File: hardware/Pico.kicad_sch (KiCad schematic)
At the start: 36 parts, among them J1 Conn_01x03 2.54mm, J5 Conn_01x04, J6 Conn_01x06, J7 Conn_01x12, U10 SRV05-4, U6 SRV05-4, U7 SRV05-4, U9 SRV05-4

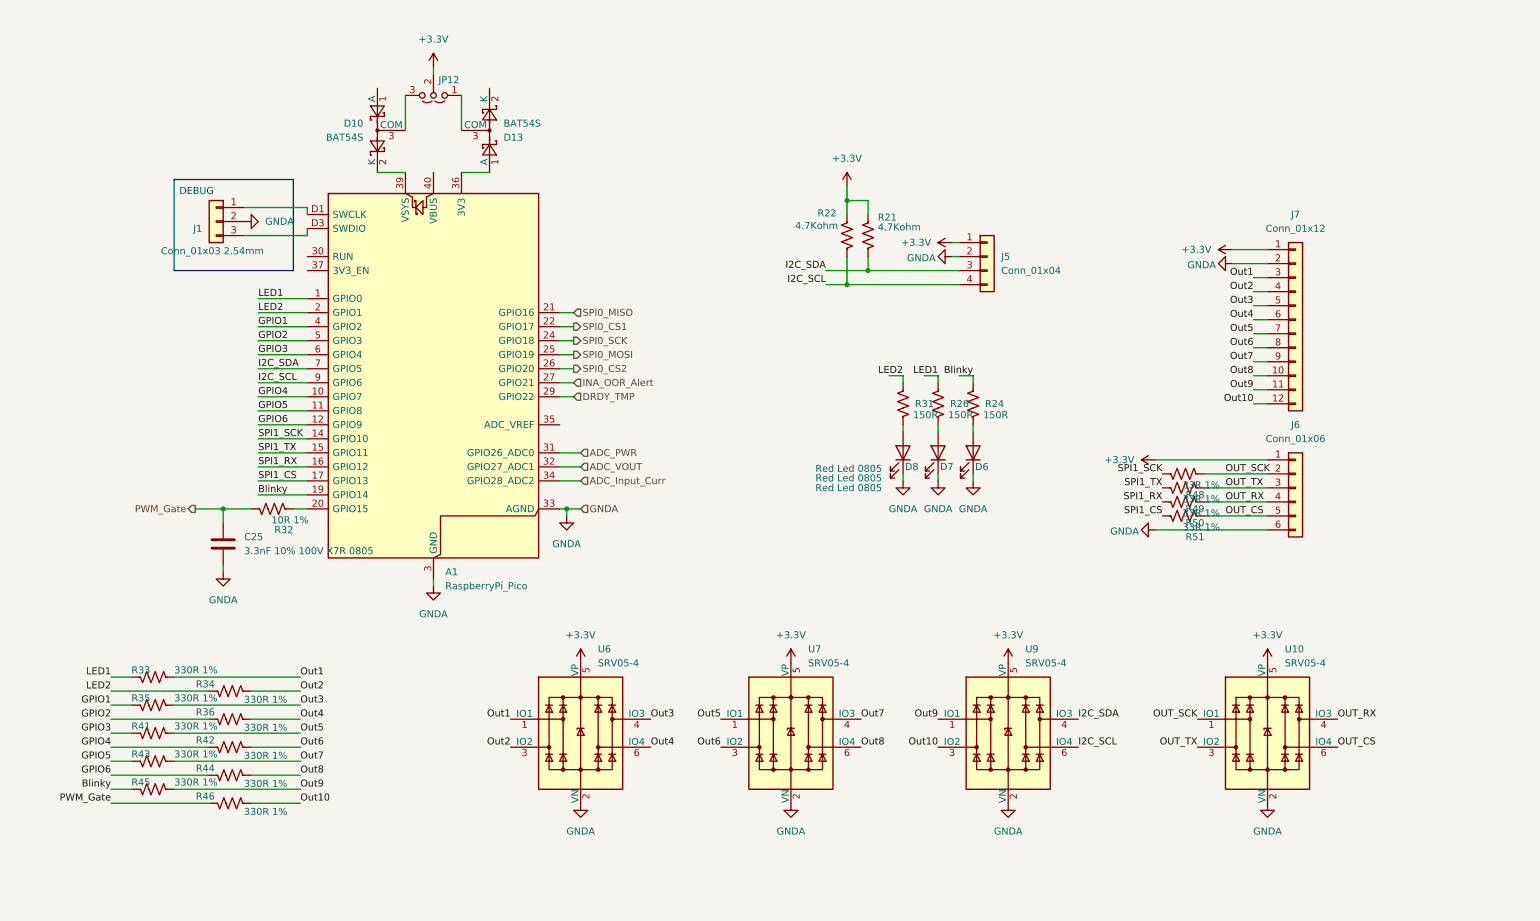
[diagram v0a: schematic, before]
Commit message: Hw/placa sepic (#34)
Co-authored-by: Federico Borello <156438142+fborello-lambda@users.noreply.github.com>
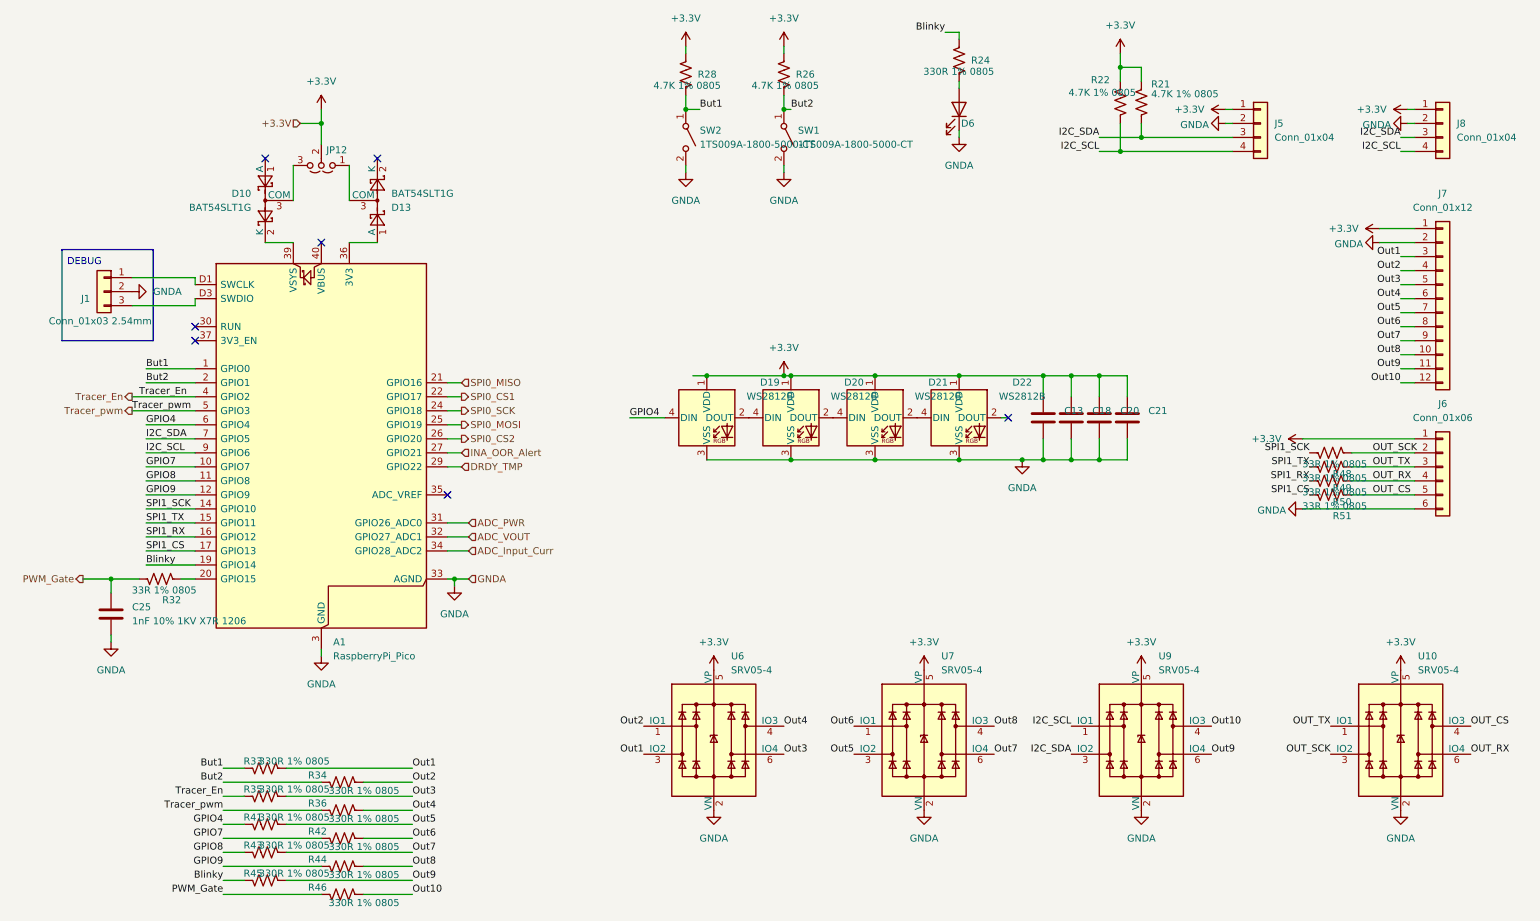
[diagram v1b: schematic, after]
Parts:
- removed D7, D8: Red Led 0805, LED_SMD:LED_0805_2012Metric_Pad1.15x1.40mm_HandSolder, symbol Device:LED
- removed R31: 150R, Resistor_SMD:R_0805_2012Metric_Pad1.20x1.40mm_HandSolder, symbol Device:R_US
- added C13, C18, C20, C21: 100nF 10% 50V X7R 0805, Capacitor_SMD:C_0805_2012Metric, symbol Device:C
- added D19, D20, D21, D22: WS2812B, LED_SMD:LED_WS2812B_PLCC4_5.0x5.0mm_P3.2mm, symbol LED:WS2812B
- added J8: Conn_01x04, Connector_PinHeader_2.54mm:PinHeader_1x04_P2.54mm_Vertical, symbol Connector_Generic:Conn_01x04
- added R28: 4.7K 1% 0805, Resistor_SMD:R_0805_2012Metric, symbol Device:R_US
- added SW1, SW2: 1TS009A-1800-5000-CT, Button_Switch_SMD:SW_Push_1TS009xxxx-xxxx-xxxx_6x6x5mm, symbol Switch:SW_SPST
- C25: value 3.3nF 10% 100V X7R 0805 -> 1nF 10% 1KV X7R 1206; footprint Capacitor_SMD:C_0805_2012Metric_Pad1.18x1.45mm_HandSolder -> Capacitor_SMD:C_1206_3216Metric
- D10, D13: value BAT54S -> BAT54SLT1G
- D6: value Red Led 0805 -> YLED0805 Red; footprint LED_SMD:LED_0805_2012Metric_Pad1.15x1.40mm_HandSolder -> LED_SMD:LED_0805_2012Metric; LCSC Part C19171391 -> (none)
- J1, JP12: LCSC Part C42431836 -> (none)
- R21, R22: value 4.7Kohm -> 4.7K 1% 0805; footprint Resistor_SMD:R_0805_2012Metric_Pad1.20x1.40mm_HandSolder -> Resistor_SMD:R_0805_2012Metric; LCSC Part C153298 -> (none)
- R24: value 150R -> 330R 1% 0805; footprint Resistor_SMD:R_0805_2012Metric_Pad1.20x1.40mm_HandSolder -> Resistor_SMD:R_0805_2012Metric; LCSC Part C153298 -> (none)
- R26: value 150R -> 4.7K 1% 0805; footprint Resistor_SMD:R_0805_2012Metric_Pad1.20x1.40mm_HandSolder -> Resistor_SMD:R_0805_2012Metric; LCSC Part C153298 -> (none)
- R32: value 10R 1% -> 33R 1% 0805; footprint Resistor_SMD:R_0805_2012Metric_Pad1.20x1.40mm_HandSolder -> Resistor_SMD:R_0805_2012Metric
- R33, R34, R35, R36, R41, R42, R43, R44, R45, R46: value 330R 1% -> 330R 1% 0805; footprint Resistor_SMD:R_0805_2012Metric_Pad1.20x1.40mm_HandSolder -> Resistor_SMD:R_0805_2012Metric
- R48, R49, R50, R51: value 33R 1% -> 33R 1% 0805; footprint Resistor_SMD:R_0805_2012Metric_Pad1.20x1.40mm_HandSolder -> Resistor_SMD:R_0805_2012Metric
- U10, U6, U7, U9: LCSC Part (none) -> C1975211
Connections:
- net GPIO3 is gone; now on net GPIO4: A1.6 (GPIO4), R41.1
- net LED2 is gone; now on net But2: A1.2 (GPIO1), R34.1
- net +3.3V: now also R26.1, C13.1, C18.1, C20.1, C21.1, D19.1 (VDD), D20.1 (VDD), D21.1 (VDD), D22.1 (VDD), J8.1 (Pin_1), R28.1
- net GNDA: now also C13.2, C18.2, C20.2, C21.2, D19.3 (VSS), D20.3 (VSS), D21.3 (VSS), D22.3 (VSS), J8.2 (Pin_2), SW1.2 (B), SW2.2 (B)
- net GPIO4: now also D19.4 (DIN); no longer A1.10 (GPIO7), R42.1
- net I2C_SCL: now also U9.1 (IO1), J8.4 (Pin_4); no longer U9.6 (IO4)
- net I2C_SDA: now also U9.3 (IO2), J8.3 (Pin_3); no longer U9.4 (IO3)
- net OUT_CS: now also U10.4 (IO3); no longer U10.6 (IO4)
- net OUT_RX: now also U10.6 (IO4); no longer U10.4 (IO3)
- net OUT_SCK: now also U10.3 (IO2); no longer U10.1 (IO1)
- net OUT_TX: now also U10.1 (IO1); no longer U10.3 (IO2)
- net Out1: now also U6.3 (IO2); no longer U6.1 (IO1)
- net Out10: now also U9.4 (IO3); no longer U9.3 (IO2)
- net Out2: now also U6.1 (IO1); no longer U6.3 (IO2)
- net Out3: now also U6.6 (IO4); no longer U6.4 (IO3)
- net Out4: now also U6.4 (IO3); no longer U6.6 (IO4)
- net Out5: now also U7.3 (IO2); no longer U7.1 (IO1)
- net Out6: now also U7.1 (IO1); no longer U7.3 (IO2)
- net Out7: now also U7.6 (IO4); no longer U7.4 (IO3)
- net Out8: now also U7.4 (IO3); no longer U7.6 (IO4)
- net Out9: now also U9.6 (IO4); no longer U9.1 (IO1)
- net But2: now reaches R26.2
- net But2: now also SW1.1 (A)
- net GPIO1 renamed Tracer_En
- net GPIO2 renamed Tracer_pwm
- net GPIO5 renamed GPIO8
- net GPIO6 renamed GPIO9
- net LED1 renamed But1
- net But1: now also R28.2, SW2.1 (A); no longer R26.1
- new net: D20.2 (DOUT), D21.4 (DIN)
- new net: D19.2 (DOUT), D20.4 (DIN)
- new net: D21.2 (DOUT), D22.4 (DIN)
- new net GPIO7: A1.10 (GPIO7), R42.1
- no-connect marks 0 -> 7
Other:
- moved on the sheet: A1, C25, D10, D13, D6, J1, J5, J6, J7, JP12, R21, R22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
